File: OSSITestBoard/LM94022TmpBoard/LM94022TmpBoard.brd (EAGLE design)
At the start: 10.2 x 21.6 mm, 8 parts, among them U1 LM94022, X1 P-PAD-S, X2 P-PAD-S, X3 P-PAD-S

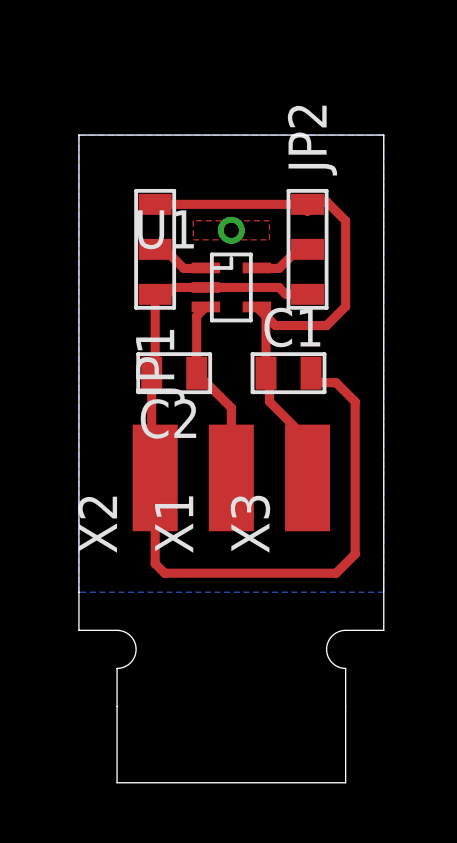
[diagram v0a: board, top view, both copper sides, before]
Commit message: temp board file added
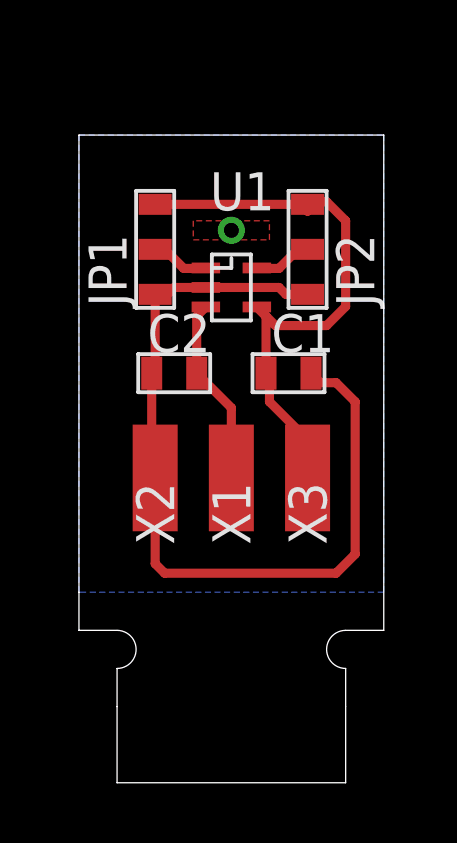
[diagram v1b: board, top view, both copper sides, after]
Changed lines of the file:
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@@
 <?xml version="1.0" encoding="utf-8"?>
 <!DOCTYPE eagle SYSTEM "eagle.dtd">
-<eagle version="6.1">
+<eagle version="6.5.0">
 <drawing>
 <settings>
@@
 <layer number="23" name="tOrigins" color="15" fill="1" visible="yes" active="yes"/>
 <layer number="24" name="bOrigins" color="15" fill="1" visible="yes" active="yes"/>
-<layer number="25" name="tNames" color="7" fill="1" visible="no" active="yes"/>
-<layer number="26" name="bNames" color="7" fill="1" visible="no" active="yes"/>
+<layer number="25" name="tNames" color="7" fill="1" visible="yes" active="yes"/>
+<layer number="26" name="bNames" color="7" fill="1" visible="yes" active="yes"/>
 <layer number="27" name="tValues" color="7" fill="1" visible="no" active="yes"/>
 <layer number="28" name="bValues" color="7" fill="1" visible="no" active="yes"/>
-<layer number="29" name="tStop" color="7" fill="3" visible="yes" active="yes"/>
-<layer number="30" name="bStop" color="7" fill="6" visible="yes" active="yes"/>
+<layer number="29" name="tStop" color="7" fill="3" visible="no" active="yes"/>
+<layer number="30" name="bStop" color="7" fill="6" visible="no" active="yes"/>
 <layer number="31" name="tCream" color="7" fill="4" visible="no" active="yes"/>
 <layer number="32" name="bCream" color="7" fill="5" visible="no" active="yes"/>
@@
 </class>
 </classes>
-<designrules>
+<designrules name="default">
 <description language="de">&lt;b&gt;EAGLE Design Rules&lt;/b&gt;
 &lt;p&gt;
@@
 </autorouter>
 <elements>
-<element name="U1" library="OSSI" package="SC70-5" value="LM94022" x="5.08" y="16.51" rot="R270"/>
-<element name="C1" library="OSSI" package="C0603(1608)" value="100nF" x="6.985" y="13.6525"/>
-<element name="JP1" library="OSSI" package="JP2SMD0603" value="JP2" x="2.54" y="17.78" rot="R270"/>
-<element name="JP2" library="OSSI" package="JP2SMD0603" value="JP2" x="7.62" y="17.78" rot="R90"/>
-<element name="C2" library="OSSI" package="C0603(1608)" value="100nF" x="3.175" y="13.6525" rot="R180"/>
-<element name="X1" library="OSSI" package="P-PAD-S" value="P-PAD-S" x="5.08" y="10.16" rot="R90"/>
-<element name="X2" library="OSSI" package="P-PAD-S" value="P-PAD-S" x="2.54" y="10.16" rot="R90"/>
-<element name="X3" library="OSSI" package="P-PAD-S" value="P-PAD-S" x="7.62" y="10.16" rot="R90"/>
+<element name="U1" library="OSSI" package="SC70-5" value="LM94022" x="5.08" y="16.51" smashed="yes" rot="R270">
+<attribute name="NAME" x="4.37" y="19.08" size="1.27" layer="25" font="vector"/>
+<attribute name="VALUE" x="1.18" y="13.91" size="1.27" layer="27"/>
+</element>
+<element name="C1" library="OSSI" package="C0603(1608)" value="100nF" x="6.985" y="13.6525" smashed="yes">
+<attribute name="NAME" x="8.509" y="15.621" size="1.27" layer="25" font="vector" rot="R180"/>
+<attribute name="VALUE" x="6.096" y="11.6205" size="1.27" layer="27"/>
+</element>
+<element name="JP1" library="OSSI" package="JP2SMD0603" value="JP2" x="2.54" y="17.78" smashed="yes" rot="R270">
+<attribute name="NAME" x="1.5875" y="15.875" size="1.27" layer="25" font="vector" rot="R90"/>
+</element>
+<element name="JP2" library="OSSI" package="JP2SMD0603" value="JP2" x="7.62" y="17.78" smashed="yes" rot="R90">
+<attribute name="NAME" x="9.8425" y="15.875" size="1.27" layer="25" font="vector" rot="R90"/>
+</element>
+<element name="C2" library="OSSI" package="C0603(1608)" value="100nF" x="3.175" y="13.6525" smashed="yes" rot="R180">
+<attribute name="NAME" x="4.3815" y="15.621" size="1.27" layer="25" font="vector" rot="R180"/>
+<attribute name="VALUE" x="4.064" y="15.6845" size="1.27" layer="27" rot="R180"/>
+</element>
+<element name="X1" library="OSSI" package="P-PAD-S" value="P-PAD-S" x="5.08" y="10.16" smashed="yes" rot="R90">
+<attribute name="NAME" x="5.715" y="7.9375" size="1.27" layer="25" font="vector" rot="R90"/>
+<attribute name="VALUE" x="7.62" y="7.62" size="1.27" layer="27" rot="R90"/>
+</element>
+<element name="X2" library="OSSI" package="P-PAD-S" value="P-PAD-S" x="2.54" y="10.16" smashed="yes" rot="R90">
+<attribute name="NAME" x="3.175" y="7.9375" size="1.27" layer="25" font="vector" rot="R90"/>
+<attribute name="VALUE" x="5.08" y="7.62" size="1.27" layer="27" rot="R90"/>
+</element>
+<element name="X3" library="OSSI" package="P-PAD-S" value="P-PAD-S" x="7.62" y="10.16" smashed="yes" rot="R90">
+<attribute name="NAME" x="8.255" y="7.9375" size="1.27" layer="25" font="vector" rot="R90"/>
+<attribute name="VALUE" x="10.16" y="7.62" size="1.27" layer="27" rot="R90"/>
+</element>
 </elements>
 <signals>
